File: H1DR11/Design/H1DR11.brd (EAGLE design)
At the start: 34.6 x 30 mm, 34 parts, among them P1 HEXABIT_17.32_NO_P6, U1 STM32F091CBU6, U2 MAX14840EASAT, X1 XTALL_CSTCE8M00G52

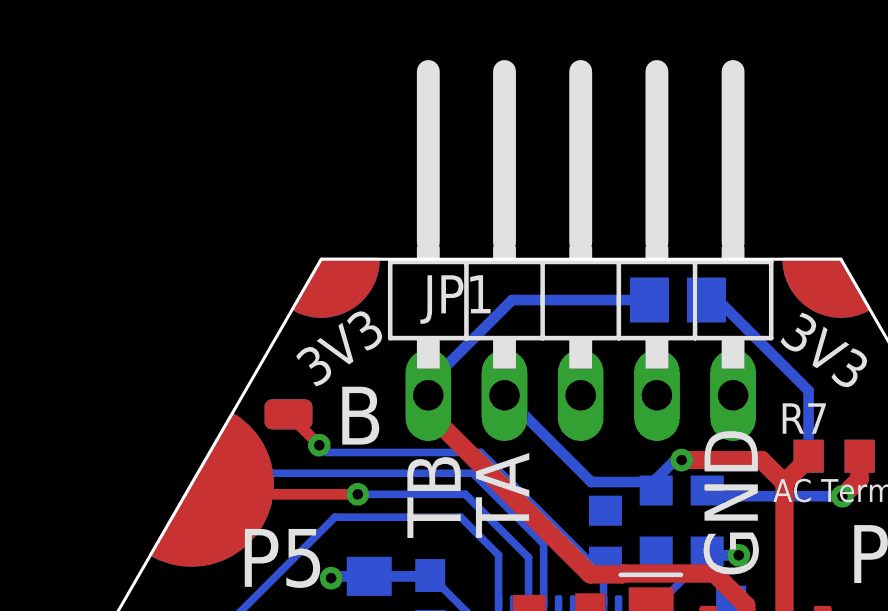
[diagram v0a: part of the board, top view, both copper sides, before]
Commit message: output CAM files generated
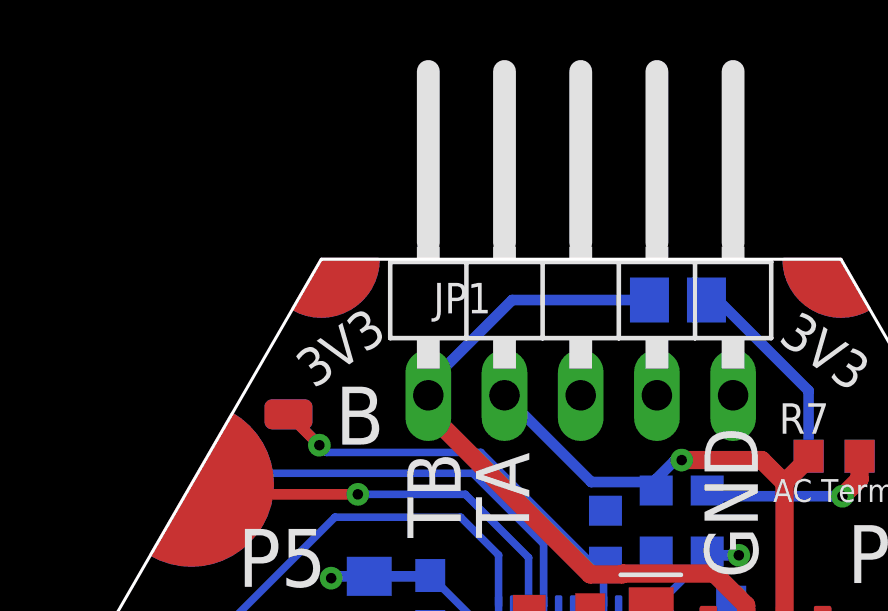
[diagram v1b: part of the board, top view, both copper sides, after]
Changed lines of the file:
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@@
 <?xml version="1.0" encoding="utf-8"?>
 <!DOCTYPE eagle SYSTEM "eagle.dtd">
-<eagle version="9.6.0">
+<eagle version="9.6.1">
 <drawing>
 <settings>
@@
 </layers>
 <board>
+<fusionsync huburn="a.cGVyc29uYWw6dWUyYWRmNjYx" projecturn="a.cGVyc29uYWw6dWUyYWRmNjYxIzIwMjAwNDI4MjkyMjA3NzAx" f3durn="urn:adsk.wipprod:dm.lineage:0bZKyB_8Qeyj0L_032PeSA" pcbguid="a5c2f18c-d076-412a-8650-0f549dc6bdb3" lastpulledtime="" lastsyncedchangeguid="" latestrevisionid="fd9aabbc-0468-4404-8163-9c2b3434560e" lastsyncedrevisionid="fd9aabbc-0468-4404-8163-9c2b3434560e" lastboardhashguid="c8d83414-8a95-2411-081f-f96d024df18d" lastpushedtime="2020-05-04T08:58:15Z" linktopcb3d="%12"/>
 <plain>
 <text x="27.3867875" y="43.37405625" size="1.9304" layer="26" rot="MR0">B</text>
@@
 </element>
 <element name="JP1" library="Hexabitz" package="1X05/90" package3d_urn="urn:adsk.eagle:package:22467/2" value="" x="34.6075" y="48.895" smashed="yes">
-<attribute name="NAME" x="31.75" y="49.0855" size="1.27" layer="25" ratio="10" rot="R180"/>
+<attribute name="DESCRIPTION" value="Conn Header R/a 5POS 2.54MM MALE" x="34.6075" y="48.895" size="1.778" layer="27" display="off"/>
+<attribute name="MFN" value="Sullins" x="34.6075" y="48.895" size="1.778" layer="27" display="off"/>
+<attribute name="MPN" value="PEC05SBAN" x="34.6075" y="48.895" size="1.778" layer="27" display="off"/>
+<attribute name="NAME" x="31.623" y="48.8315" size="1.016" layer="25" ratio="10" rot="R180"/>
+<attribute name="OCTOPART_URL" value="https://octopart.com/pec05sban-sullins-264498?r=sp" x="34.6075" y="48.895" size="1.778" layer="27" display="off"/>
 <attribute name="POPULARITY" value="9" x="34.6075" y="48.895" size="1.778" layer="27" display="off"/>
 <attribute name="VALUE" x="42.8625" y="45.085" size="1.27" layer="27" rot="R90"/>
@@
 <compatibility>
 <note version="8.3" severity="warning">
+Since Version 8.3, EAGLE supports Fusion synchronisation.
+This feature will not be available in this version and saving
+the document will break the link to the Fusion PCB feature.
+</note>
+<note version="8.3" severity="warning">
 Since Version 8.3, EAGLE supports URNs for individual library
